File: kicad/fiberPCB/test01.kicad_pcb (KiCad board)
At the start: 2 copper layers, 33 x 24 mm, 23 parts, among them J1 Conn_01x01_Male, J2 Conn_01x01_Male, J3 Conn_01x01_Male, J4 Conn_01x01_Male, J5 Conn_01x01_Male, J6 Conn_01x01_Male, J7 Conn_01x01_Male, J8 Conn_01x01_Male, P5 Conn_01x10_Male

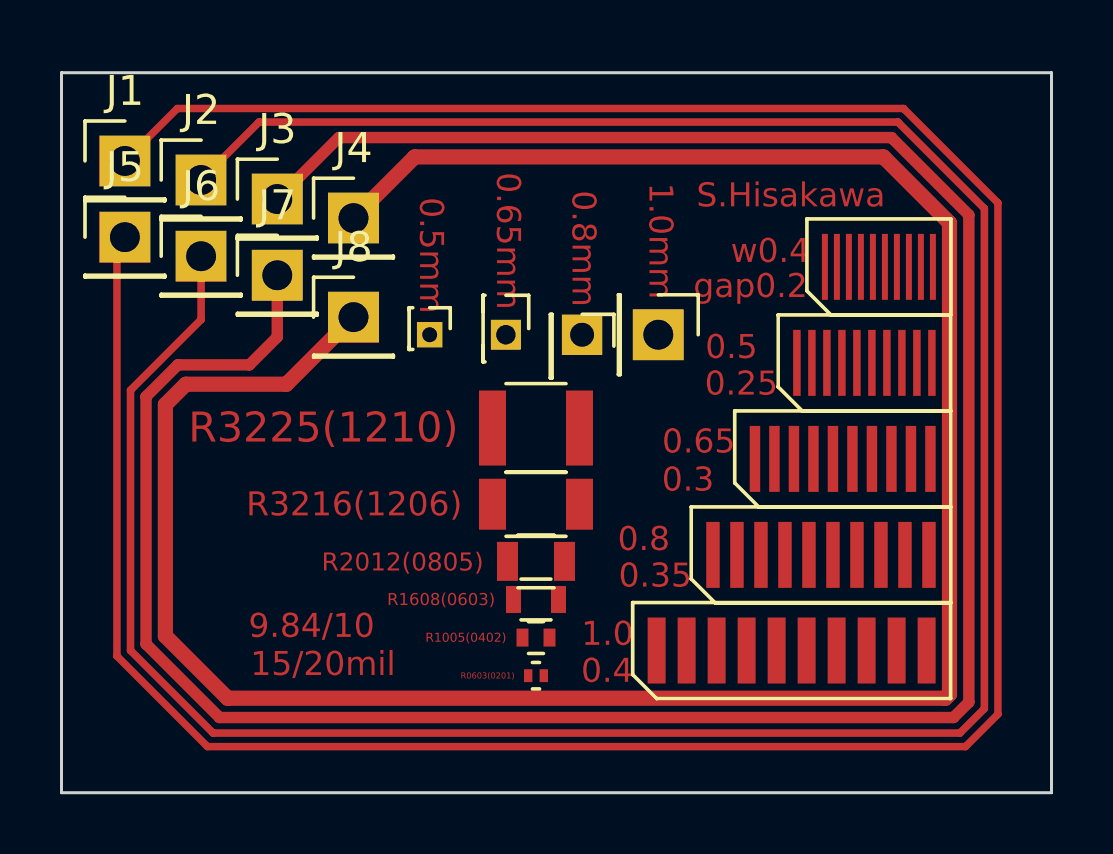
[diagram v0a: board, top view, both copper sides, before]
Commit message: made test01 pattern
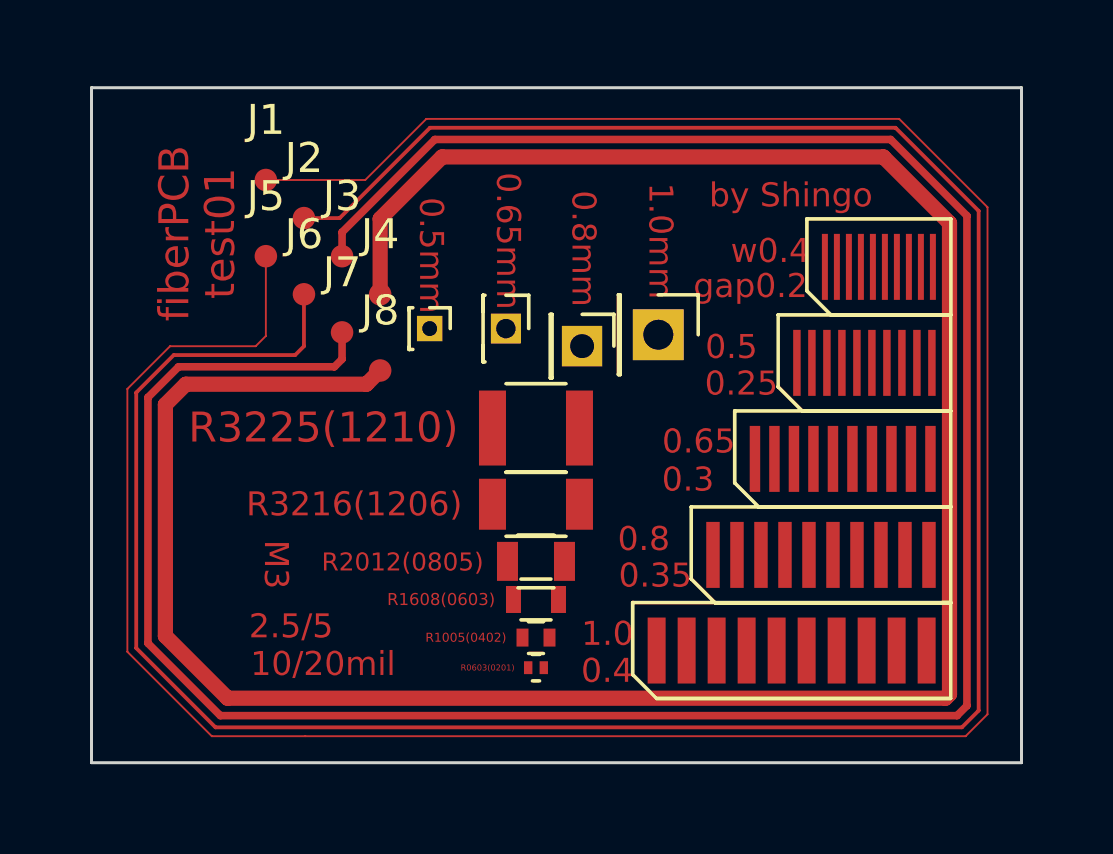
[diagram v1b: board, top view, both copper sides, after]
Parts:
- J1, J2, J3, J4, J5, J6, J7, J8: footprint Pin_Headers:Pin_Header_Straight_1x01_Pitch2.54mm -> fiberPCB:Checkpoint
- moved J1 4.74 mm to (146.8, 36.6)
- moved J5 4.74 mm to (146.8, 39.1)
- moved J6 3.66 mm to (148.1, 40.4)
- moved J2 3.66 mm to (148.1, 37.8)
- moved J3 2.88 mm to (149.4, 39.1)
- moved J7 2.88 mm to (149.4, 41.7)
- moved J4 2.69 mm to (150.6, 40.4)
- moved J8 1.99 mm to (150.6, 42.9)
- moved R0603(0201) 0.27 mm to (155.8, 52.8)
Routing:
- net Net-(J1-Pad1): track 93.3 -> 89.9 mm
- net Net-(J4-Pad1): track 79.6 -> 81.4 mm
- net Net-(J2-Pad1): track 88.8 -> 87.4 mm
- net Net-(J3-Pad1): track 85.4 -> 84.8 mm
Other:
- board size 33 x 24 mm -> 31 x 22.5 mm
- rule trace_min: 0.2 -> 0.0254
- rule via_min_size: 0.4 -> 0.0254
- board text added: "10/20mil"
- board text added: "2.5/5"
- board text added: "22.5x31mm"
- board text added: "M3"
- board text added: "by Shingo"
- board text added: "fiberPCB"
- board text added: "test01"
- board text removed: "15/20mil"
- board text removed: "24x33mm"
- board text removed: "9.84/10"
- board text removed: "S.Hisakawa"
